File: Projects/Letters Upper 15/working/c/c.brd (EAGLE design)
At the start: 16.5 x 21.6 mm, 42 parts

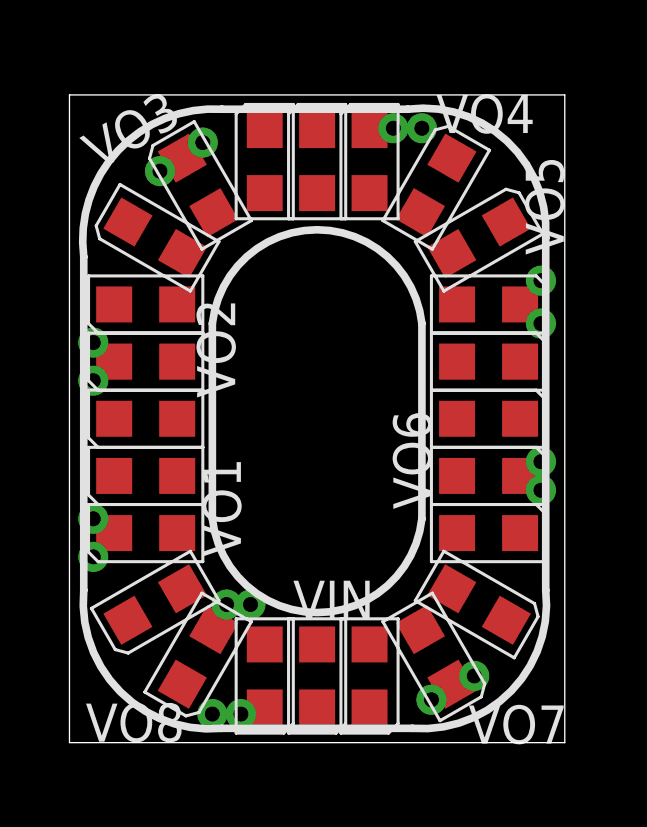
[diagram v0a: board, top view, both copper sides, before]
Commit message: continued working.
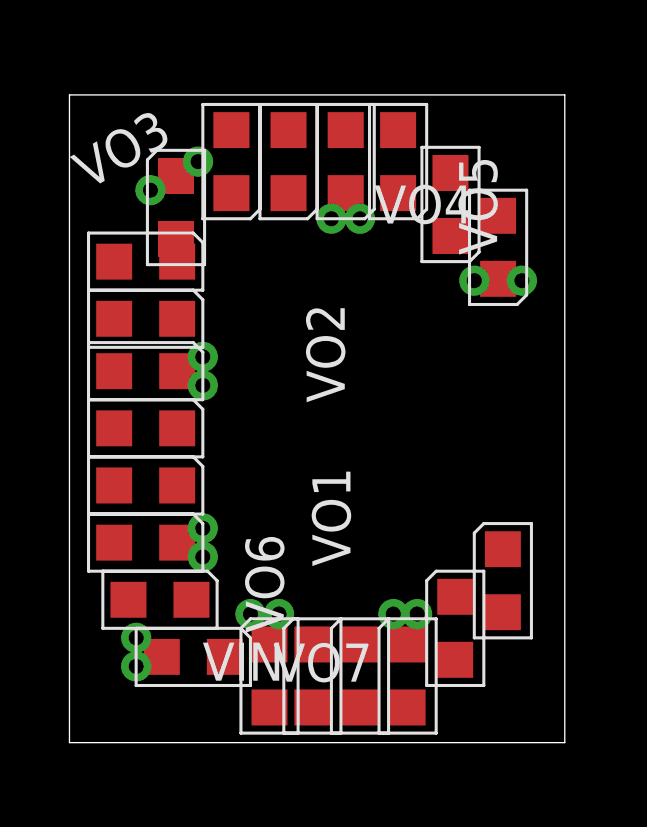
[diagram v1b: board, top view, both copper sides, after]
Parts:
- removed LED22, LED23, LED24: (no value), CyberRailGuru:LED_0805
- removed VO15, VO16: (no value), CyberRailGuru:P1-20
- moved VO14 10.9 mm to (6.03, 4.29)
- moved VO13 10.5 mm to (11.6, 4.29)
- moved VO9 7.60 mm to (4.45, 12.9)
- moved LED16 7.32 mm to (14.4, 5.40), turned to 0 degrees
- moved LED18 7.19 mm to (11.3, 2.22), turned to 0 degrees
- moved LED17 7.07 mm to (12.9, 3.81), turned to 0 degrees
- moved VO10 6.97 mm to (4.29, 19.4)
- moved VO7 6.83 mm to (6.99, 4.29)
- moved VO12 6.65 mm to (15.1, 15.4)
- moved VO6 6.42 mm to (10.8, 4.29)
- moved LED19 6.41 mm to (9.68, 2.22), turned to 0 degrees
- moved LED20 6.05 mm to (8.10, 2.22), turned to 0 degrees
- moved LED21 5.59 mm to (6.67, 2.22), turned to 0 degrees
- moved VO8 5.39 mm to (4.45, 6.19)
- moved VO11 4.98 mm to (8.73, 17.5)
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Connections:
- removed net N$1: LED22.C, LED23.A
- removed net N$2: LED23.C, LED24.A
- removed net N$5: LED24.C, VO16.TP, VO8.TP
- net VIN: no longer LED22.A
- net VOUT1: now also VO8.TP; no longer VO9.TP
- net VOUT2: now also VO9.TP; no longer VO10.TP
- net VOUT3: now also VO10.TP; no longer VO11.TP
- net VOUT4: now also VO11.TP; no longer VO12.TP
- net VOUT5: now also VO12.TP; no longer VO13.TP
- net VOUT6: now also VO13.TP; no longer VO14.TP
- net VOUT7: now also VO14.TP; no longer VO15.TP
